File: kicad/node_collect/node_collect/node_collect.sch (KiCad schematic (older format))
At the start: 5 parts

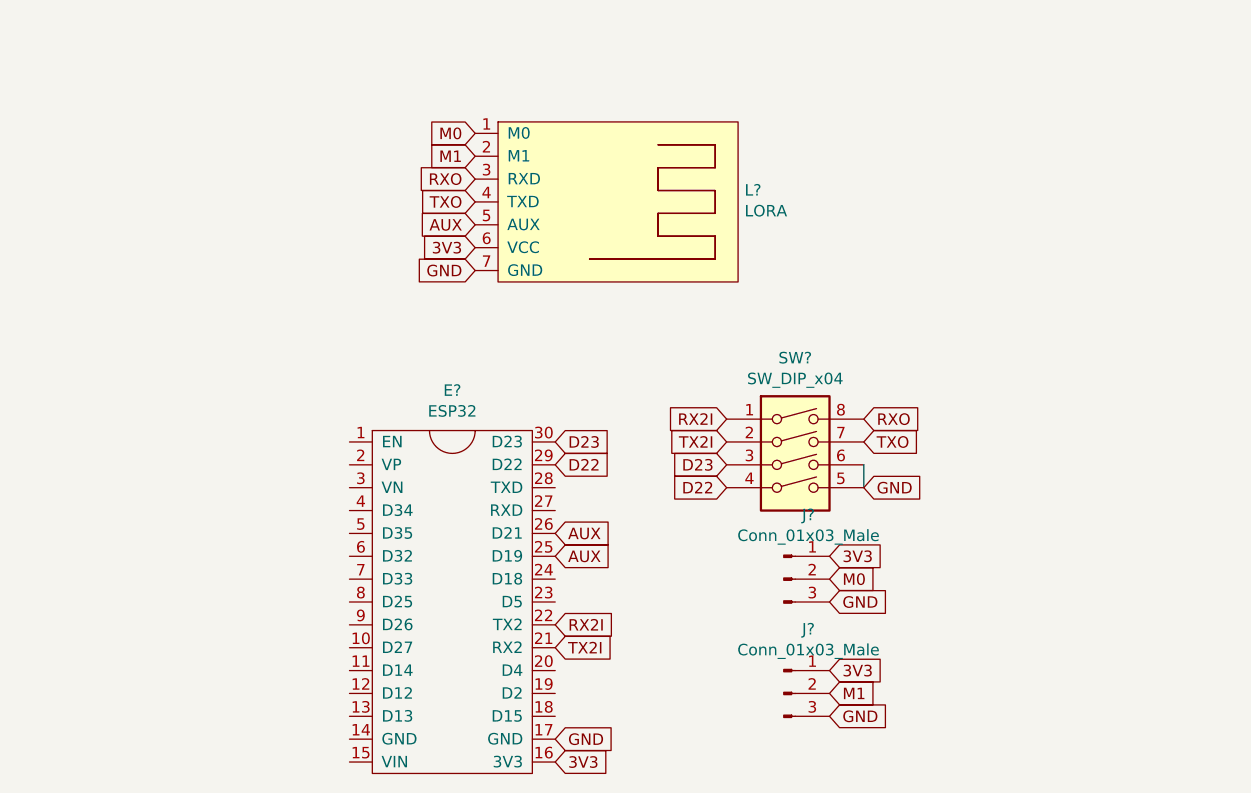
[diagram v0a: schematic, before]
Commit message: 3698
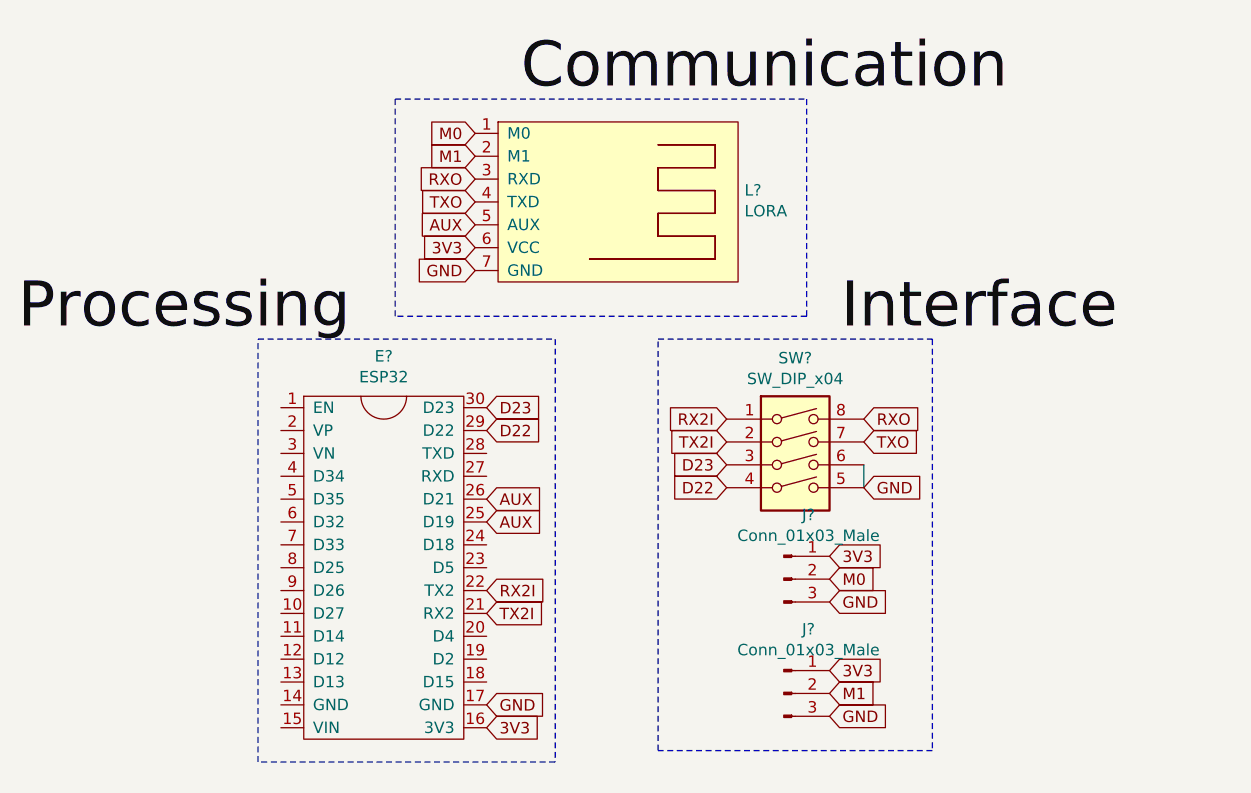
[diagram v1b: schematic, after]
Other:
- moved on the sheet: E?
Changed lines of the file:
@@
 L custom:ESP32 E?
 U 1 1 5F8E2DAF
-P 5350 4250
-F 0 "E?" H 5350 4925 50  0000 C CNN
-F 1 "ESP32" H 5350 4834 50  0000 C CNN
-F 2 "" H 5350 3200 50  0001 C CNN
-F 3 "" H 5350 3200 50  0001 C CNN
-	1    5350 4250
+P 5050 4100
+F 0 "E?" H 5050 4775 50  0000 C CNN
+F 1 "ESP32" H 5050 4684 50  0000 C CNN
+F 2 "" H 5050 3050 50  0001 C CNN
+F 3 "" H 5050 3050 50  0001 C CNN
+	1    5050 4100
 	1    0    0    -1
 $EndComp
@@
 	1    0    0    -1
 $EndComp
-Text GLabel 5800 4700 2    50   Input ~ 0
+Text GLabel 5500 4550 2    50   Input ~ 0
 TX2I
-Text GLabel 5800 4600 2    50   Input ~ 0
+Text GLabel 5500 4450 2    50   Input ~ 0
 RX2I
-Text GLabel 5800 5100 2    50   Input ~ 0
+Text GLabel 5500 4950 2    50   Input ~ 0
 GND
 Text GLabel 6550 3700 0    50   Input ~ 0
@@
 Text GLabel 6550 3800 0    50   Input ~ 0
 TX2I
-Text GLabel 5800 3800 2    50   Input ~ 0
+Text GLabel 5500 3650 2    50   Input ~ 0
 D23
 Text GLabel 6550 3900 0    50   Input ~ 0
@@
 Text GLabel 6550 4000 0    50   Input ~ 0
 D22
-Text GLabel 5800 3900 2    50   Input ~ 0
+Text GLabel 5500 3750 2    50   Input ~ 0
 D22
 Text GLabel 5450 2650 0    50   Input ~ 0
@@
 Wire Wire Line
 	7150 3900 7150 4000
-Text GLabel 5800 5200 2    50   Input ~ 0
+Text GLabel 5500 5050 2    50   Input ~ 0
 3V3
 $Comp
@@
 Text GLabel 5450 2550 0    50   Input ~ 0
 M1
-Text GLabel 5800 4200 2    50   Input ~ 0
+Text GLabel 5500 4050 2    50   Input ~ 0
 AUX
-Text GLabel 5800 4300 2    50   Input ~ 0
+Text GLabel 5500 4150 2    50   Input ~ 0
 AUX
 Text GLabel 5450 2850 0    50   Input ~ 0
@@
 Text GLabel 7150 4000 2    50   Input ~ 0
 GND
+Wire Notes Line
+	5100 2300 6900 2300
+Wire Notes Line
+	6900 2300 6900 3250
+Wire Notes Line
+	6900 3250 5100 3250
+Wire Notes Line
+	5100 3250 5100 2300
+Wire Notes Line
+	4500 3350 5800 3350
+Wire Notes Line
+	5800 3350 5800 5200
+Wire Notes Line
+	5800 5200 4500 5200
+Wire Notes Line
+	4500 5200 4500 3350
+Wire Notes Line
+	6250 3350 7450 3350
+Wire Notes Line
+	7450 3350 7450 5150
+Wire Notes Line
+	7450 5150 6250 5150
+Wire Notes Line
+	6250 5150 6250 3350
+Text Label 5650 2300 0    197  ~ 0
+Communication
+Text Label 7050 3350 0    197  ~ 0
+Interface
+Text Label 3450 3350 0    197  ~ 0
+Processing
 $EndSCHEMATC
